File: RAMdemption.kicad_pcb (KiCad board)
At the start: 4 copper layers, 99 x 53.5 mm, 41 parts, among them J1 Conn_RAM_Expansion, U1 TC518512FTL-70, U10 TC518512FTL-70, U11 TC518512FTL-70, U12 TC518512FTL-70, U13 TC518512FTL-70, U14 TC518512FTL-70, U15 TC518512FTL-70, U16 TC518512FTL-70, U17 TC518512FTL-70, U18 TC518512FTL-70, U19 TC518512FTL-70, U2 TC518512FTL-70, U20 TC518512FTL-70, U3 TC518512FTL-70, U4 TC518512FTL-70, U5 TC518512FTL-70, U6 TC518512FTL-70, U7 TC518512FTL-70, U8 TC518512FTL-70, U9 TC518512FTL-70

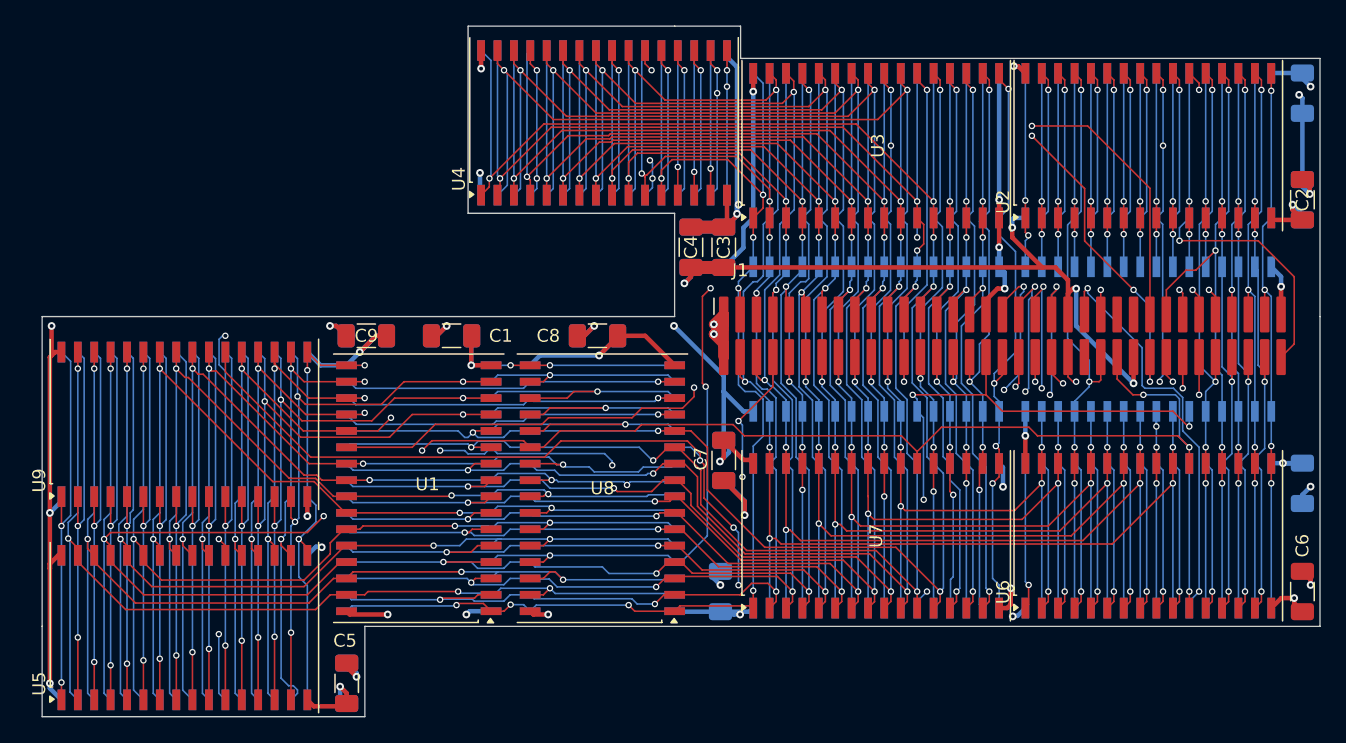
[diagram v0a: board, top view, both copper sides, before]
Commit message: routing complete
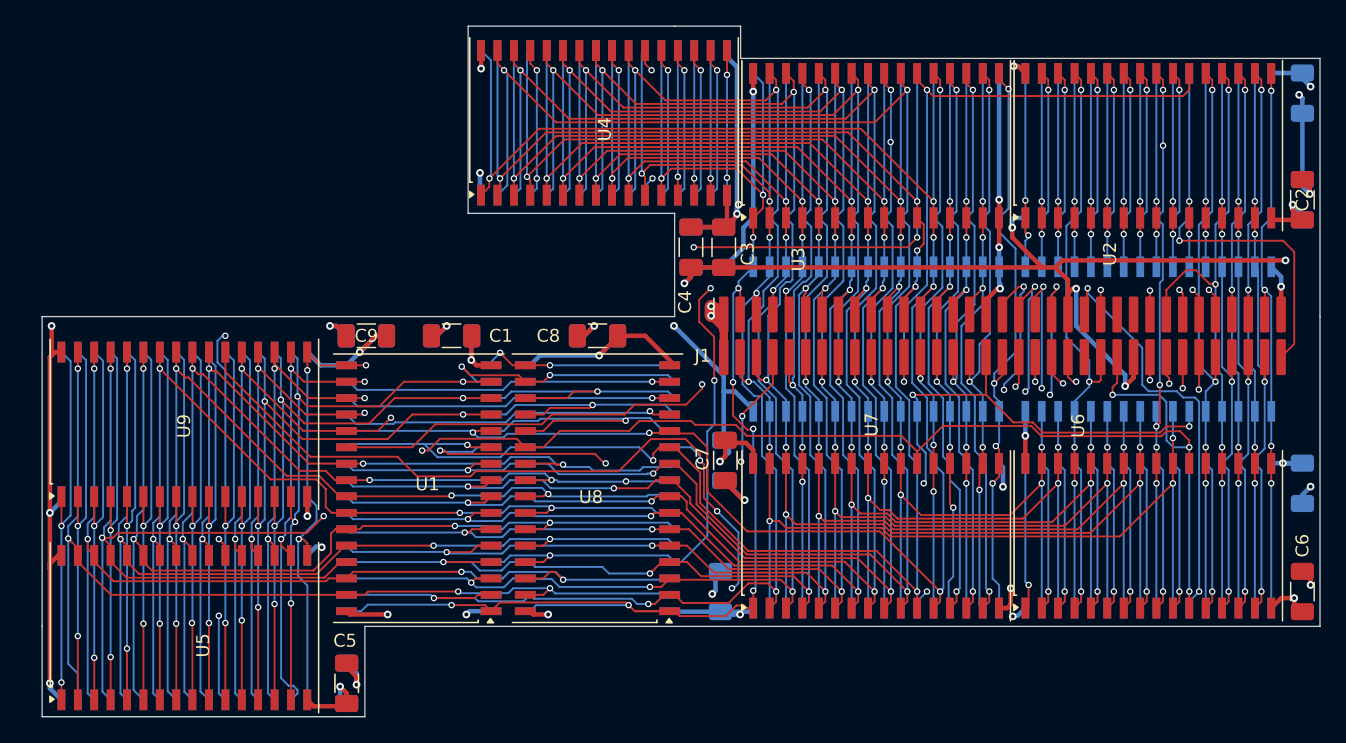
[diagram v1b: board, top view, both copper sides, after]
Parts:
- U10, U14, U18, U2, U6: footprint RAMdemption:TSOP-II-32_Repinned -> RAMdemption:TSOP-II-32_ReversedAddr
- U12, U16, U8: footprint Package_SO:TSOP-II-32_21.0x10.2mm_P1.27mm -> RAMdemption:TSOP-II-NormalAddr-Data3
- U20, U4: footprint RAMdemption:TSOP-II-32_Repinned -> RAMdemption:TSOP-II-32_ReversedAddr_Data3
- moved U12 0.38 mm to (89.9, 69.6)
- moved U8 0.38 mm to (89.9, 69.6)
- moved C7 0.13 mm to (99.8, 67.4)
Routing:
- net /RAM Bank 1/D31: track 36.8 -> 150.7 mm
- net /RAM Bank 1/D29: track 33.8 -> 147.5 mm
- net /RAM Bank 1/D30: track 34.7 -> 147.3 mm
- net /RAM Bank 1/D28: track 78.5 -> 144.9 mm, vias 6 -> 3
- net /RAM Bank 1/D26: track 83.3 -> 136.9 mm
- net /RAM Bank 1/D25: track 82.7 -> 134.5 mm
- net /RAM Bank 1/D24: track 82.7 -> 133.5 mm, vias 3 -> 4
- net /RAM Bank 1/D27: track 71.2 -> 117.2 mm
- net ~{CS6}: track 131.8 -> 124.8 mm
- net /RAM Bank 1/A18: track 267.5 -> 273.5 mm, vias 13 -> 14
- net GND: track 127.8 -> 123.0 mm
- net /RAM Bank 1/A0: track 250.0 -> 245.2 mm
- net +5V: track 519.9 -> 515.2 mm, vias 27 -> 28
- net /RAM Bank 1/A16: track 268.5 -> 264.3 mm
- net /RAM Bank 1/A2: track 252.9 -> 248.8 mm
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
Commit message: various improvements
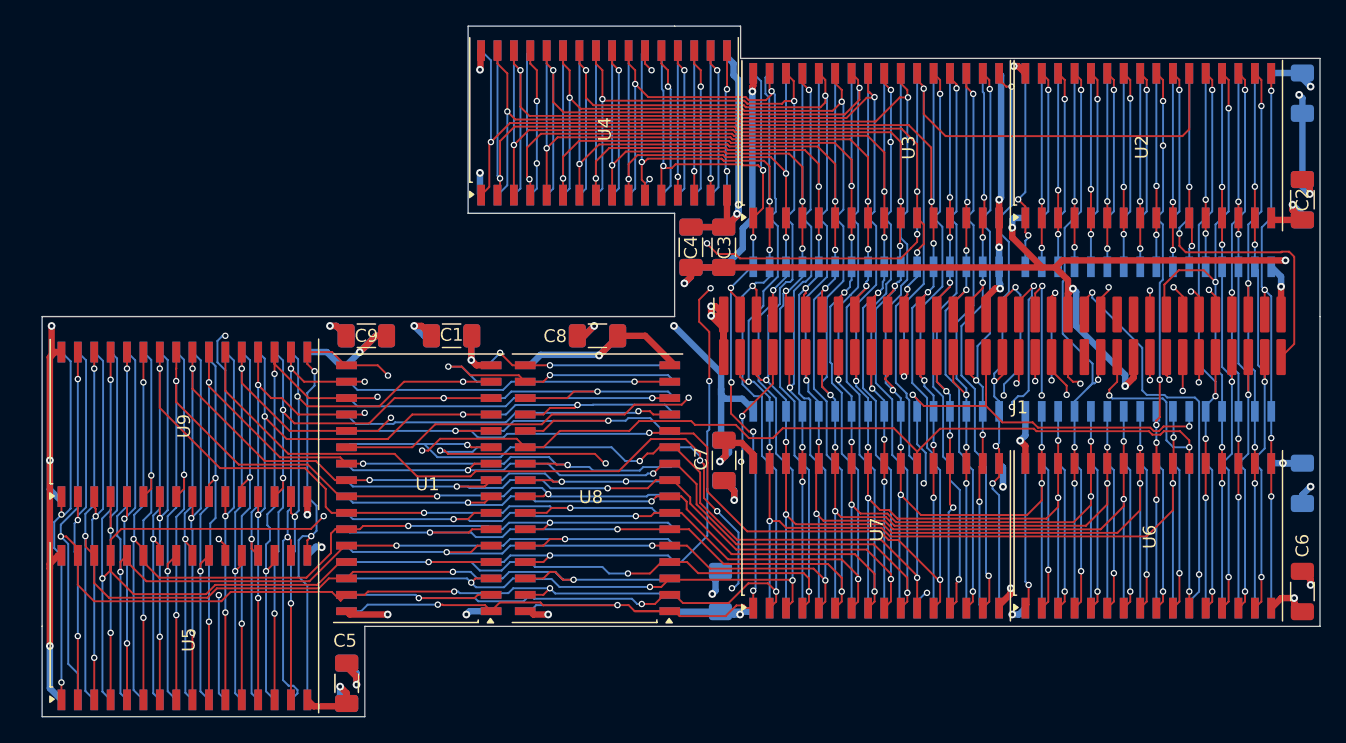
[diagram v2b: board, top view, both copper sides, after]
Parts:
- moved C7 0.10 mm to (99.7, 67.4)
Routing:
- net +5V: track 515.2 -> 524.8 mm
- net /RAM Bank 1/A16: track 264.3 -> 271.6 mm
- net /RAM Bank 1/A12: track 260.7 -> 267.9 mm
- net /RAM Bank 1/A4: track 253.9 -> 260.5 mm
- net /RAM Bank 1/A6: track 257.9 -> 264.4 mm
- net /RAM Bank 1/A15: track 261.1 -> 266.8 mm
- net /RAM Bank 1/A2: track 248.8 -> 254.3 mm
- net ~{CS2}: track 119.0 -> 123.4 mm
- net /RAM Bank 1/A9: track 249.8 -> 254.1 mm
- net /RAM Bank 1/D24: track 133.5 -> 137.3 mm
- net /~{WE0}: track 112.6 -> 116.0 mm
- net /RAM Bank 1/A17: track 257.9 -> 261.1 mm
- net /RAM Bank 1/A13: track 253.4 -> 256.5 mm
- net ~{CS6}: track 124.8 -> 127.7 mm
- net ~{OE}: track 238.1 -> 240.7 mm
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
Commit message: fix drc
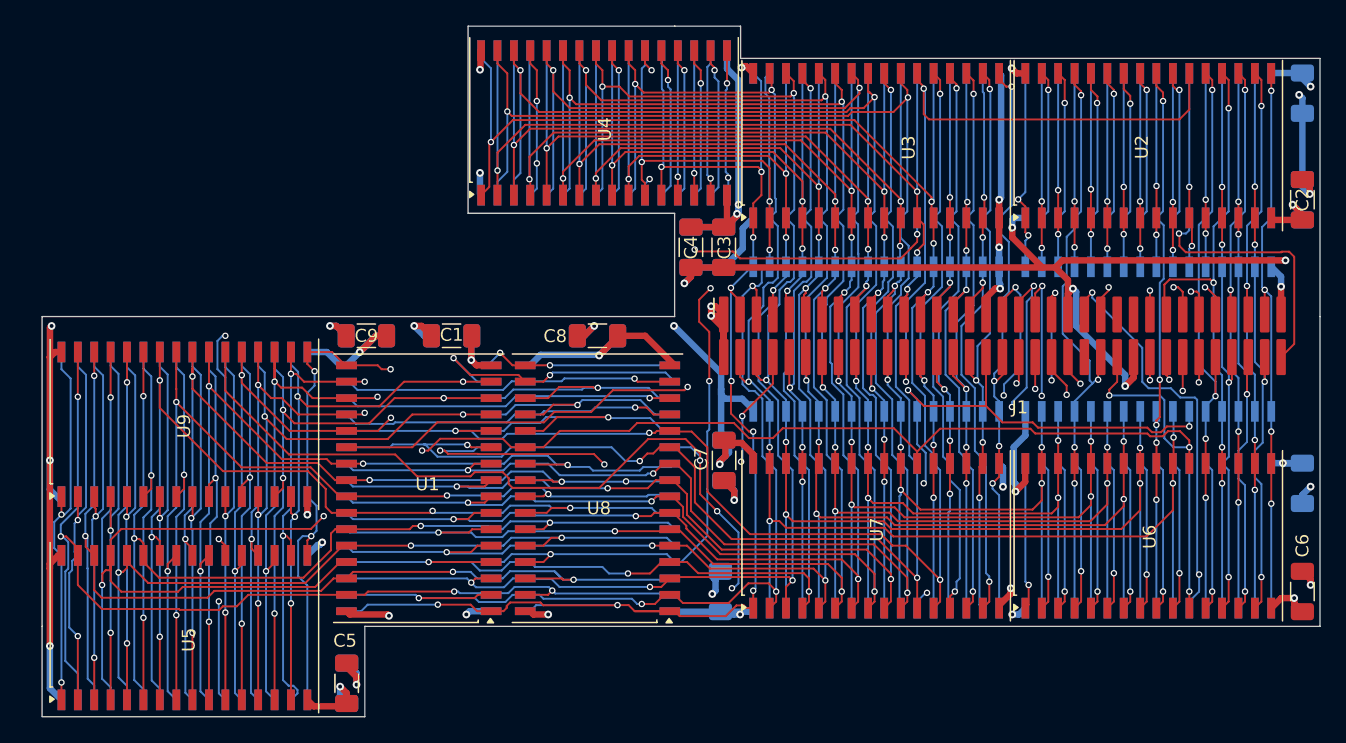
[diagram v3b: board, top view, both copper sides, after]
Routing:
- net +5V: track 524.8 -> 539.2 mm
- net /RAM Bank 1/A1: track 255.2 -> 250.0 mm
- net /RAM Bank 1/A4: track 260.5 -> 256.3 mm
- net /RAM Bank 1/A5: track 256.7 -> 252.6 mm
- net /RAM Bank 1/A7: track 260.3 -> 256.2 mm
- net /RAM Bank 1/A0: track 246.2 -> 242.3 mm
- net /RAM Bank 1/A6: track 264.4 -> 260.6 mm
- net /RAM Bank 1/A3: track 254.7 -> 250.9 mm
- net /RAM Bank 1/D6: track 102.8 -> 99.4 mm
- net /RAM Bank 1/A2: track 254.3 -> 250.9 mm
- net /RAM Bank 1/A12: track 267.9 -> 264.9 mm
- net /RAM Bank 1/D28: track 144.6 -> 147.6 mm
- net /RAM Bank 1/A13: track 256.5 -> 254.1 mm
- net /RAM Bank 1/D30: track 147.3 -> 149.3 mm
- net /~{WE3}: track 106.8 -> 104.8 mm
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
